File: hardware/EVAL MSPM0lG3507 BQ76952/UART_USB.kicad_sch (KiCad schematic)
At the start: 11 parts, among them J16 USB_B_Micro, U1 ISO7721D, U12 FT230XS, U3 19255A33A, U4 ISO7721D

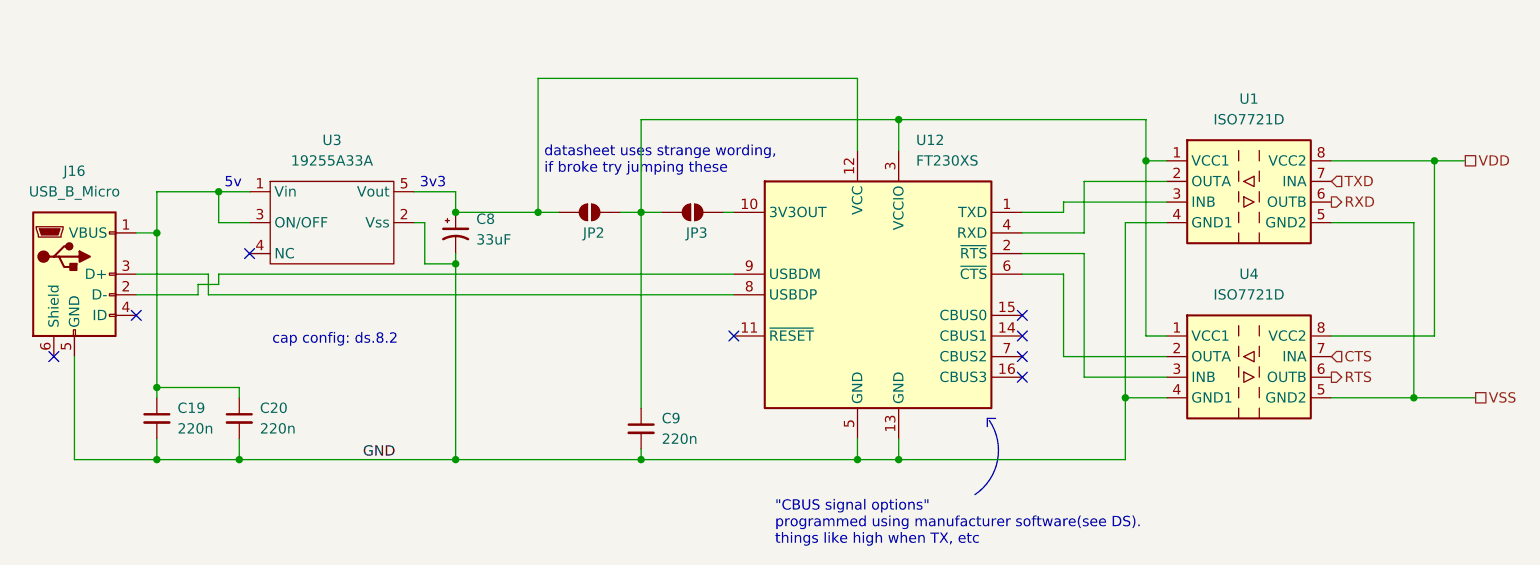
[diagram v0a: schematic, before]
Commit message: bluhhh
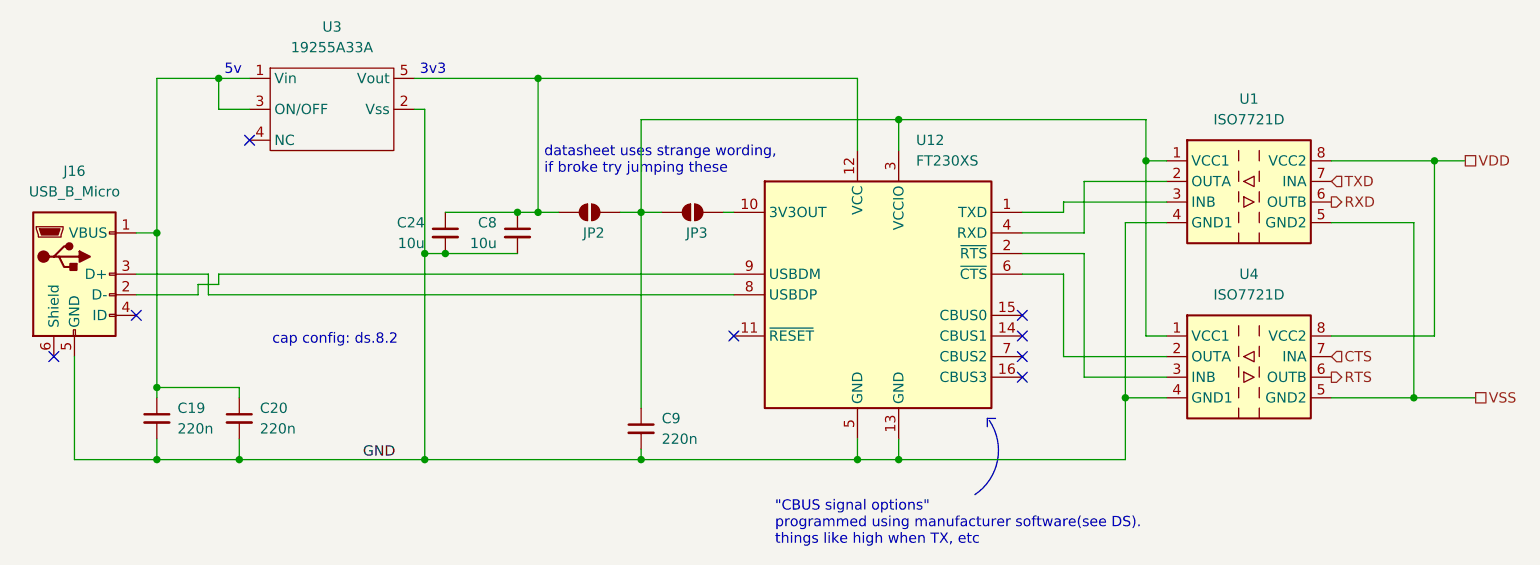
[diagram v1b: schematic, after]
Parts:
- removed C8: 33uF, Diode_SMD:D_1206_3216Metric_Pad1.42x1.75mm_HandSolder, symbol Device:C_Polarized_Small_US
- added C24, C8: 10u, Capacitor_SMD:C_1206_3216Metric_Pad1.33x1.80mm_HandSolder, symbol Device:C_Small
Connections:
- net GND: now also C24.2, C8.2
- net at JP2.2 (B), U12.12 (VCC), U3.5 (Vout): now also C24.1, C8.1
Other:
- moved on the sheet: U3
